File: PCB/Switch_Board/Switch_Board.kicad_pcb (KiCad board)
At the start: 2 copper layers, 99.8 x 99.8 mm, 15 parts, among them J1 Conn_01x04_Pin, J4 Conn_01x04_Pin

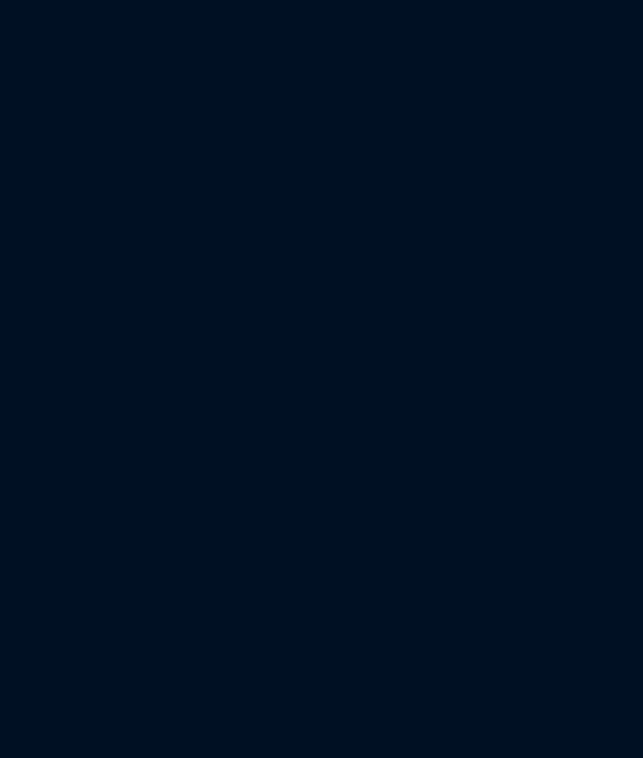
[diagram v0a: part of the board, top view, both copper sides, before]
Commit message: FINAL SWITCH BOARD
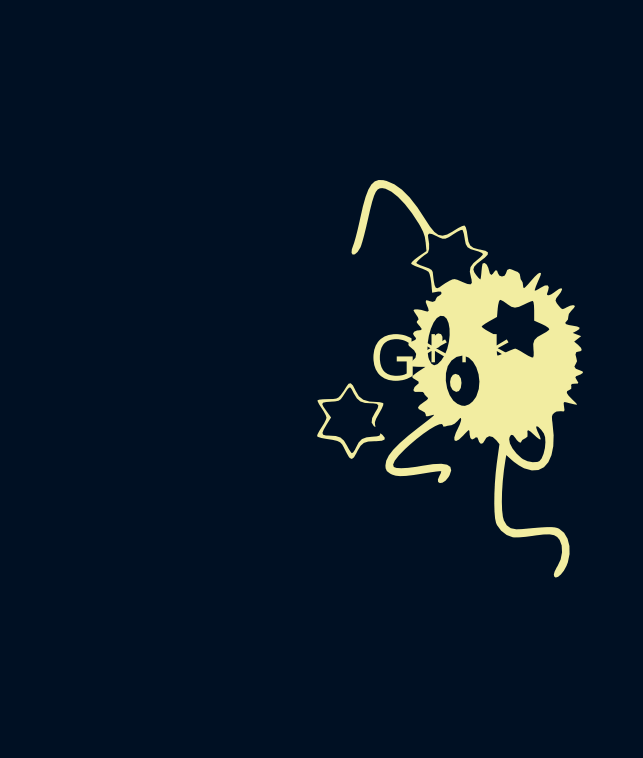
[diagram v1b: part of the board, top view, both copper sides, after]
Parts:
- added G***: LOGO, LOGO, F.Cu at (184.8, 60.0)
